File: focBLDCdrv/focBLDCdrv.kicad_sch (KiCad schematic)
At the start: 23 parts, among them J1 Screw_Terminal_01x02, J2 Screw_Terminal_01x03, J3 Conn_01x08, J4 i2c, J5 Conn_02x03_Top_Bottom, J6 Monitor port, J7 Power Out, U1 MFC8316A

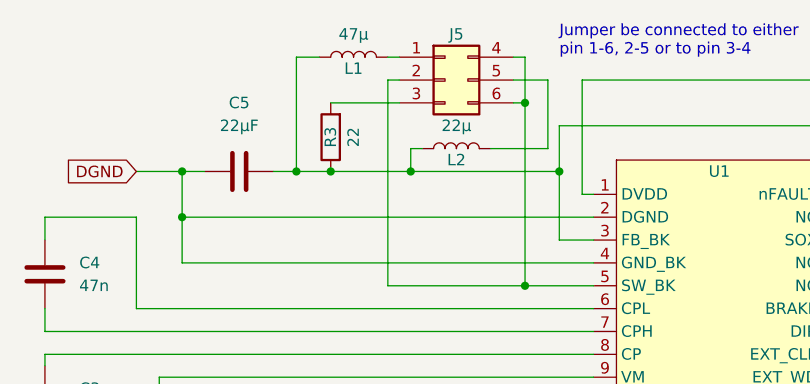
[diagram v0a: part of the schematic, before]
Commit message: Hasty checkin of current development projects...
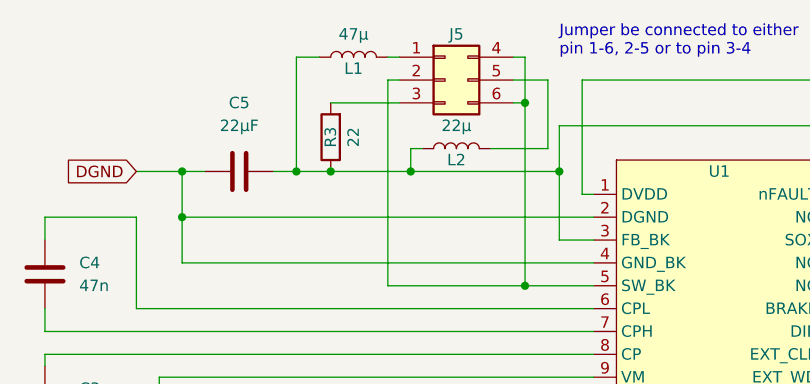
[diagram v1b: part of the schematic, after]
